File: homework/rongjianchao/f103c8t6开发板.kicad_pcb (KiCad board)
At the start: 2 copper layers, 40 x 40 mm, 45 parts, among them J1 Conn_01x04, J10 Conn_01x03, J11 Conn_01x03, J12 Conn_01x04, J13 Conn_01x04, J3 Conn_01x03, J4 Conn_01x02, J5 USB_C_Receptacle_USB2.0, J6 Conn_01x06, J7 Conn_01x04, J8 Conn_01x04, J9 Conn_01x03, SW1 SW, SW2 SW, SW3 SW, U1 STM32F103C8Tx, U3 HX9193-33GB, U4 TJA1051T-3, U5 CH340E, Y1 12M

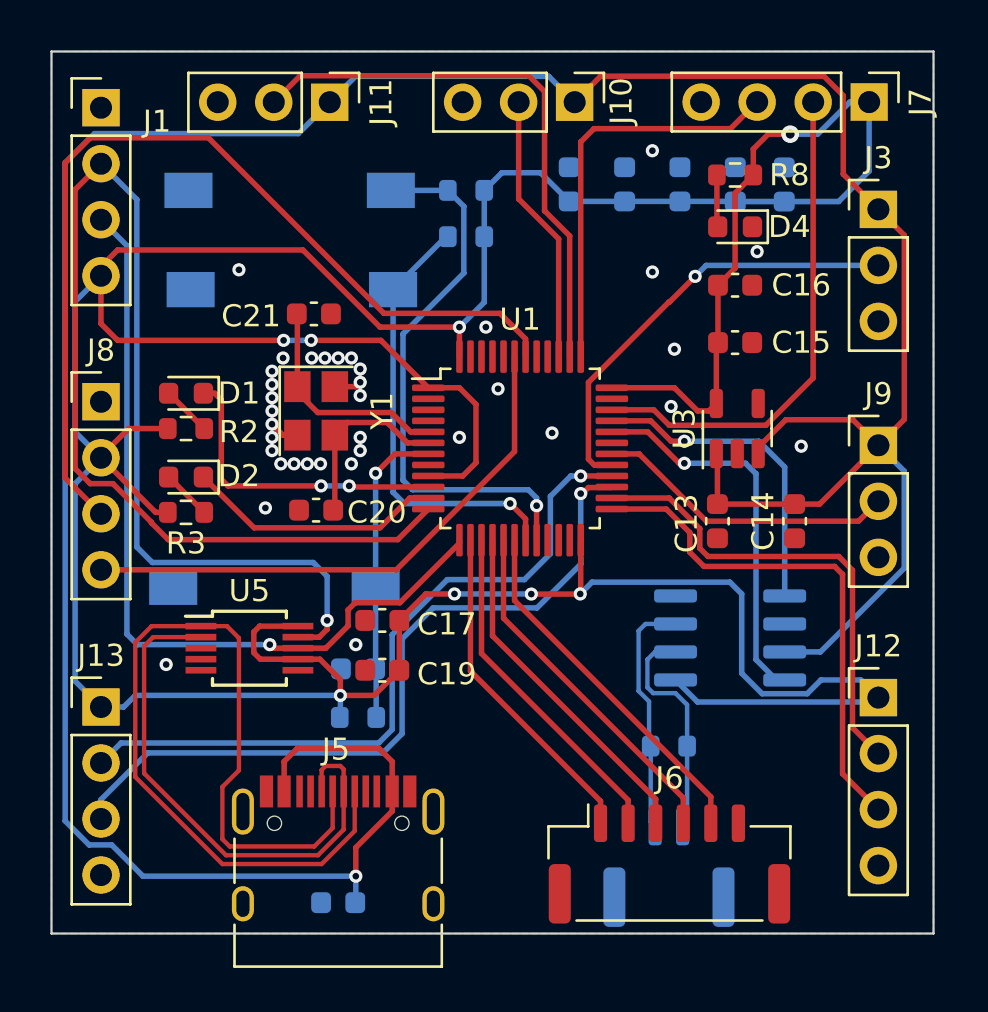
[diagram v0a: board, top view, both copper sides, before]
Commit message: 容键超2
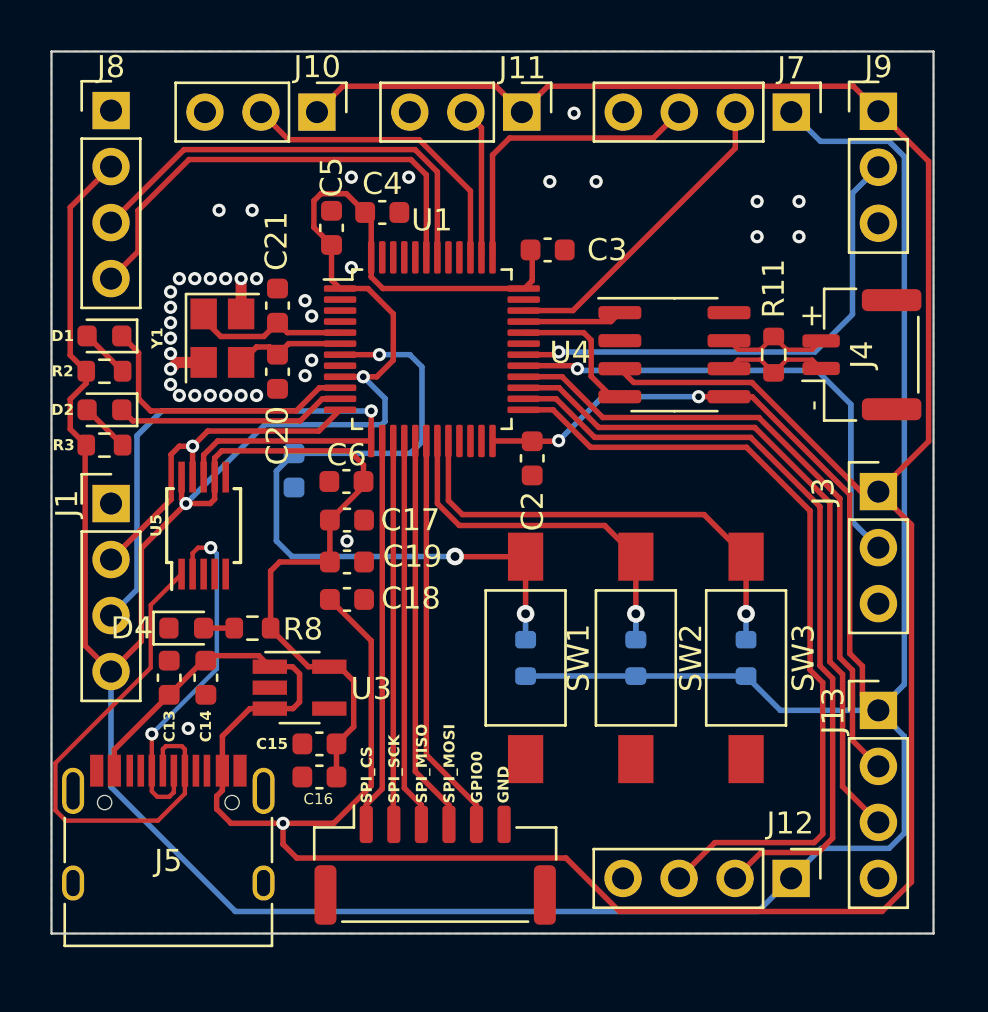
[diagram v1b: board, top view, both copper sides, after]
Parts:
- C18, C2, C3, C4, C5, C6, J4, R11, SW1, SW2, SW3, U4: moved to F.Cu
- U3: footprint PackageSOT:SOT-23-5 -> Package_TO_SOT_SMD:SOT-23-5_HandSoldering
- moved J13 35.3 mm to (217.5, 101.9)
- moved D4 30.8 mm to (186.1, 98.2), turned to 0 degrees
- moved R8 30.0 mm to (189.1, 98.2)
- moved SW3 29.6 mm to (211.5, 99.5), turned to -90 degrees
- moved C16 29.2 mm to (192.2, 104.9), turned to 0 degrees
- moved C14 27.6 mm to (187.0, 100.4)
- moved C15 26.2 mm to (192.2, 103.4), turned to 0 degrees
- moved C13 25.9 mm to (185.3, 100.4), turned to -90 degrees
- moved J4 24.8 mm to (216.8, 85.8), turned to 90 degrees
- moved R5 24.7 mm to (211.5, 99.5), turned to -90 degrees
- moved C6 24.0 mm to (193.4, 91.5), turned to 0 degrees
- moved U3 23.1 mm to (191.2, 100.8), turned to 0 degrees
- moved SW2 22.9 mm to (206.5, 99.5), turned to -90 degrees
- moved R4 20.6 mm to (206.5, 99.5), turned to -90 degrees
- moved C5 18.4 mm to (192.7, 80.0)
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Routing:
- net /Connector/TXD: track 63.4 -> 15.8 mm
- net +3V3: track 192.2 -> 234.3 mm, vias 8 -> 4
- net /Connector/I2C1_SCL: track 42.5 -> 20.5 mm
- net /MCU/RESET: track 13.9 -> 33.0 mm, vias 1 -> 3
- net /Connector/TIM2_CH1: track 25.6 -> 6.88 mm
- net /Connector/DP: track 41.9 -> 23.8 mm
- net /Connector/PB13: track 21.6 -> 35.9 mm
- net /Connector/PB12: track 23.6 -> 37.1 mm
- net /Connector/CAN_RX: track 17.4 -> 6.53 mm, vias 1 -> 0
- net /Connector/CAN_TX: track 14.5 -> 4.53 mm, vias 1 -> 0
- net /Connector/TIM1_CH2: track 13.7 -> 22.8 mm, vias 0 -> 1
- net /MCU/DIO: track 22.8 -> 14.3 mm
- net /Connector/DN: track 24.4 -> 16.4 mm, vias 0 -> 2
- net /Connector/RXD: track 37.2 -> 30.0 mm
- net /Connector/+: track 11.0 -> 5.01 mm
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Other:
- board text added: "+"
- board text added: "-"
- board text added: "GND"
- board text added: "GPIO0"
- board text added: "SPI_CS"
- board text added: "SPI_MISO"
- board text added: "SPI_MOSI"
- board text added: "SPI_SCK"
